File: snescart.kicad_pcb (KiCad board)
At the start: 2 copper layers, 101.6 x 37.3 mm, 7 parts, among them P1 CASSETTE, U1 27C080

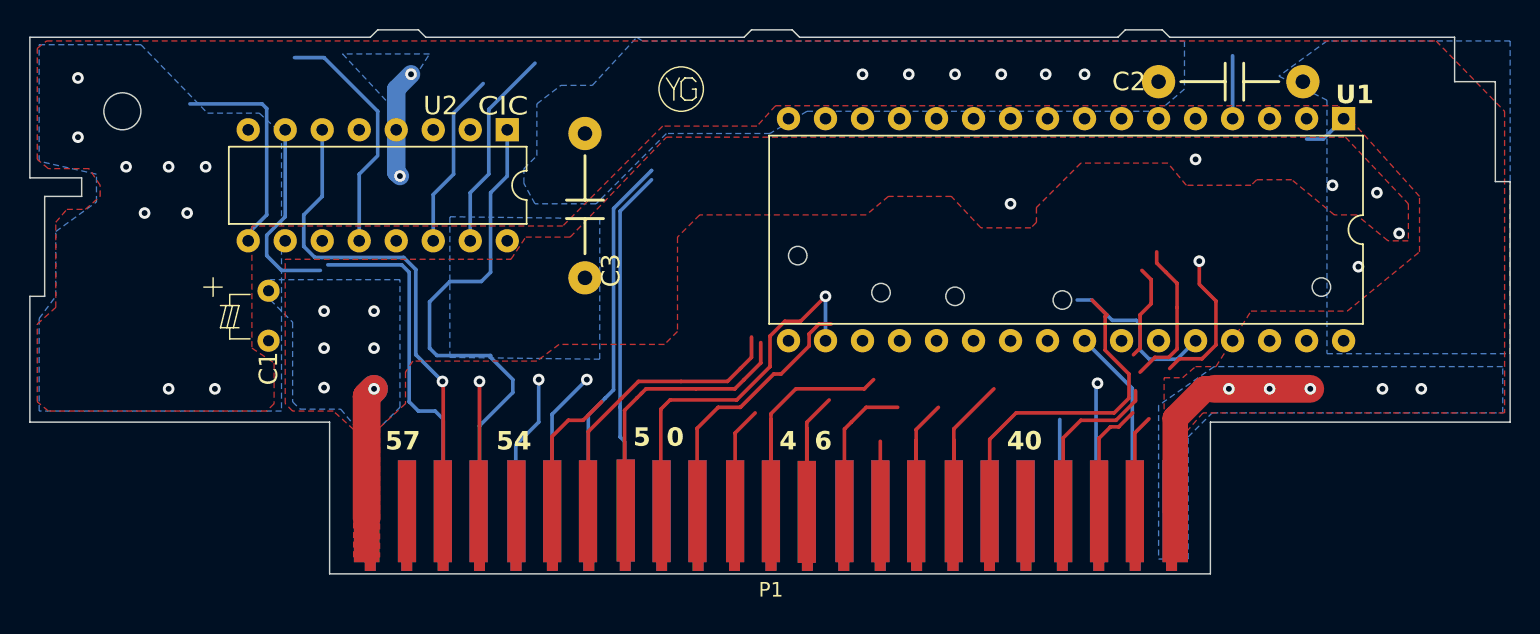
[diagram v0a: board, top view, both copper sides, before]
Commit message: ftghjdrftgh
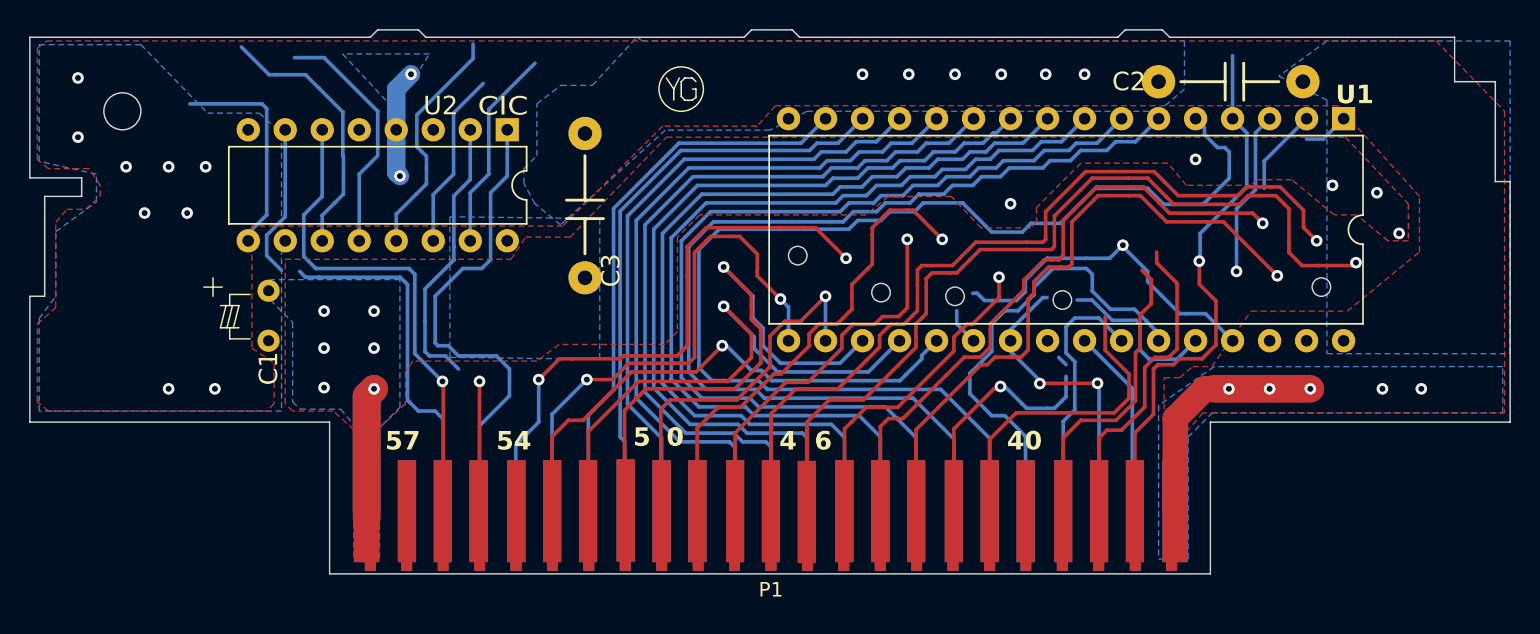
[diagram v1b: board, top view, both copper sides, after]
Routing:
- net Net-(P1-A7): track 0.00 -> 81.4 mm
- net Net-(P1-A6): track 0.00 -> 69.6 mm
- net Net-(P1-A5): track 0.00 -> 65.9 mm
- net Net-(P1-A4): track 0.00 -> 62.6 mm
- net Net-(P1-A3): track 0.00 -> 59.1 mm
- net Net-(P1-A2): track 0.00 -> 55.5 mm
- net Net-(P1-A1): track 0.00 -> 51.7 mm
- net unconnected-(P1-A21-Pad46): track 14.1 -> 65.0 mm, vias 0 -> 1
- net Net-(P1-A0): track 0.00 -> 48.3 mm
- net unconnected-(P1-A22-Pad47): track 21.0 -> 63.7 mm, vias 0 -> 1
- net Net-(P1-D0): track 0.00 -> 42.7 mm
- net Net-(P1-A19): track 7.91 -> 45.8 mm
- net Net-(P1-A18): track 12.6 -> 48.4 mm, vias 0 -> 1
- net Net-(P1-A8): track 0.00 -> 31.9 mm
- net unconnected-(P1-RD-Pad23): track 10.4 -> 40.7 mm, vias 1 -> 2
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
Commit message: sdgs
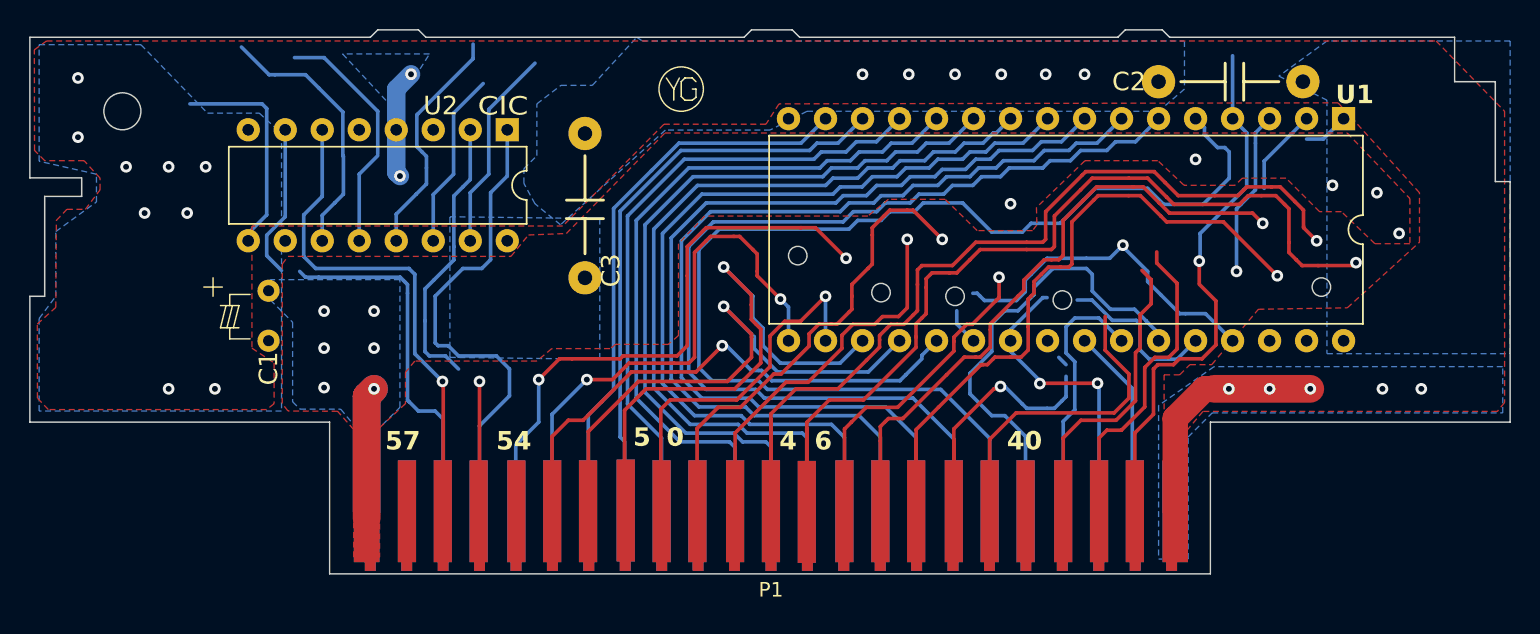
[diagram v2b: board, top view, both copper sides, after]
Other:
- board text added: "C"
- board text added: "MASK"
- board text added: "N"
- board text added: "ROM"
- board text added: "n"
- board text added: "o"
- board text removed: "MASK ROM"
